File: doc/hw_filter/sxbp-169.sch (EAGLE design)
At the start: 3 parts

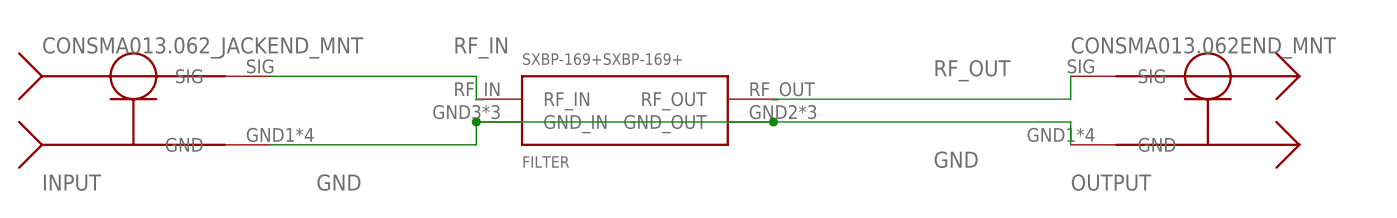
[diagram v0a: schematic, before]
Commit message: updated libraries
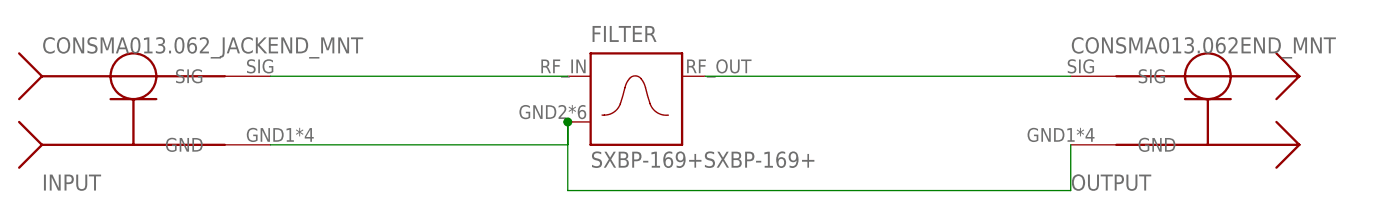
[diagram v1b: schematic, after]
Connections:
- net RF_IN renamed N$1
- net RF_OUT renamed N$3
- net GND: no longer FILTER.GND_OUT
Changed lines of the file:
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@@
 <?xml version="1.0" encoding="utf-8"?>
 <!DOCTYPE eagle SYSTEM "eagle.dtd">
-<eagle version="7.2.0">
+<eagle version="8.0.0">
 <drawing>
 <settings>
@@
 <layers>
 <layer number="1" name="Top" color="4" fill="1" visible="no" active="no"/>
+<layer number="2" name="Route2" color="1" fill="3" visible="no" active="no"/>
+<layer number="3" name="Route3" color="4" fill="3" visible="no" active="no"/>
+<layer number="4" name="Route4" color="1" fill="4" visible="no" active="no"/>
+<layer number="5" name="Route5" color="4" fill="4" visible="no" active="no"/>
+<layer number="6" name="Route6" color="1" fill="8" visible="no" active="no"/>
+<layer number="7" name="Route7" color="4" fill="8" visible="no" active="no"/>
+<layer number="8" name="Route8" color="1" fill="2" visible="no" active="no"/>
+<layer number="9" name="Route9" color="4" fill="2" visible="no" active="no"/>
+<layer number="10" name="Route10" color="1" fill="7" visible="no" active="no"/>
+<layer number="11" name="Route11" color="4" fill="7" visible="no" active="no"/>
+<layer number="12" name="Route12" color="1" fill="5" visible="no" active="no"/>
+<layer number="13" name="Route13" color="4" fill="5" visible="no" active="no"/>
+<layer number="14" name="Route14" color="1" fill="6" visible="no" active="no"/>
+<layer number="15" name="Route15" color="4" fill="6" visible="no" active="no"/>
 <layer number="16" name="Bottom" color="1" fill="1" visible="no" active="no"/>
 <layer number="17" name="Pads" color="2" fill="1" visible="no" active="no"/>
@@
 <instance part="INPUT" gate="G$1" x="-12.7" y="53.34"/>
 <instance part="OUTPUT" gate="G$1" x="106.68" y="53.34"/>
-<instance part="FILTER" gate="SXBP-169+" x="40.64" y="53.34"/>
+<instance part="FILTER" gate="SXBP-169+" x="53.34" y="58.42"/>
 </instances>
 <busses>
 </busses>
 <nets>
+<net name="N$1" class="0">
+<segment>
+<pinref part="INPUT" gate="G$1" pin="SIG"/>
+<pinref part="FILTER" gate="SXBP-169+" pin="RF_IN"/>
+<wire x1="12.7" y1="60.96" x2="45.72" y2="60.96" width="0.1524" layer="91"/>
+</segment>
+</net>
 <net name="GND" class="0">
 <segment>
 <pinref part="INPUT" gate="G$1" pin="GND"/>
-<wire x1="12.7" y1="53.34" x2="35.56" y2="53.34" width="0.1524" layer="91"/>
-<wire x1="35.56" y1="53.34" x2="35.56" y2="55.88" width="0.1524" layer="91"/>
 <pinref part="FILTER" gate="SXBP-169+" pin="GND_IN"/>
-<label x="17.78" y="48.26" size="1.778" layer="95"/>
+<wire x1="12.7" y1="53.34" x2="45.72" y2="53.34" width="0.1524" layer="91"/>
+<wire x1="45.72" y1="53.34" x2="45.72" y2="55.88" width="0.1524" layer="91"/>
+<wire x1="45.72" y1="55.88" x2="45.72" y2="48.26" width="0.1524" layer="91"/>
+<wire x1="45.72" y1="48.26" x2="101.6" y2="48.26" width="0.1524" layer="91"/>
+<junction x="45.72" y="55.88"/>
 <pinref part="OUTPUT" gate="G$1" pin="GND"/>
-<pinref part="FILTER" gate="SXBP-169+" pin="GND_OUT"/>
-<wire x1="68.58" y1="55.88" x2="101.6" y2="55.88" width="0.1524" layer="91"/>
-<wire x1="101.6" y1="55.88" x2="101.6" y2="53.34" width="0.1524" layer="91"/>
-<label x="86.36" y="50.8" size="1.778" layer="95"/>
-<wire x1="35.56" y1="55.88" x2="68.58" y2="55.88" width="0.1524" layer="91"/>
-<junction x="35.56" y="55.88"/>
-<junction x="68.58" y="55.88"/>
+<wire x1="101.6" y1="48.26" x2="101.6" y2="53.34" width="0.1524" layer="91"/>
 </segment>
 </net>
-<net name="RF_IN" class="0">
+<net name="N$3" class="0">
 <segment>
-<pinref part="INPUT" gate="G$1" pin="SIG"/>
-<wire x1="12.7" y1="60.96" x2="35.56" y2="60.96" width="0.1524" layer="91"/>
-<wire x1="35.56" y1="60.96" x2="35.56" y2="58.42" width="0.1524" layer="91"/>
-<pinref part="FILTER" gate="SXBP-169+" pin="RF_IN"/>
-<label x="33.02" y="63.5" size="1.778" layer="95"/>
+<pinref part="OUTPUT" gate="G$1" pin="SIG"/>
+<pinref part="FILTER" gate="SXBP-169+" pin="RF_OUT"/>
+<wire x1="101.6" y1="60.96" x2="60.96" y2="60.96" width="0.1524" layer="91"/>
 </segment>
 </net>
-<net name="RF_OUT" class="0">
-<segment>
-<pinref part="OUTPUT" gate="G$1" pin="SIG"/>
-<wire x1="68.58" y1="58.42" x2="101.6" y2="58.42" width="0.1524" layer="91"/>
-<wire x1="101.6" y1="58.42" x2="101.6" y2="60.96" width="0.1524" layer="91"/>
-<pinref part="FILTER" gate="SXBP-169+" pin="RF_OUT"/>
-<label x="86.36" y="60.96" size="1.778" layer="95"/>
-</segment>
-</net>
